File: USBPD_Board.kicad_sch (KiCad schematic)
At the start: 0 parts

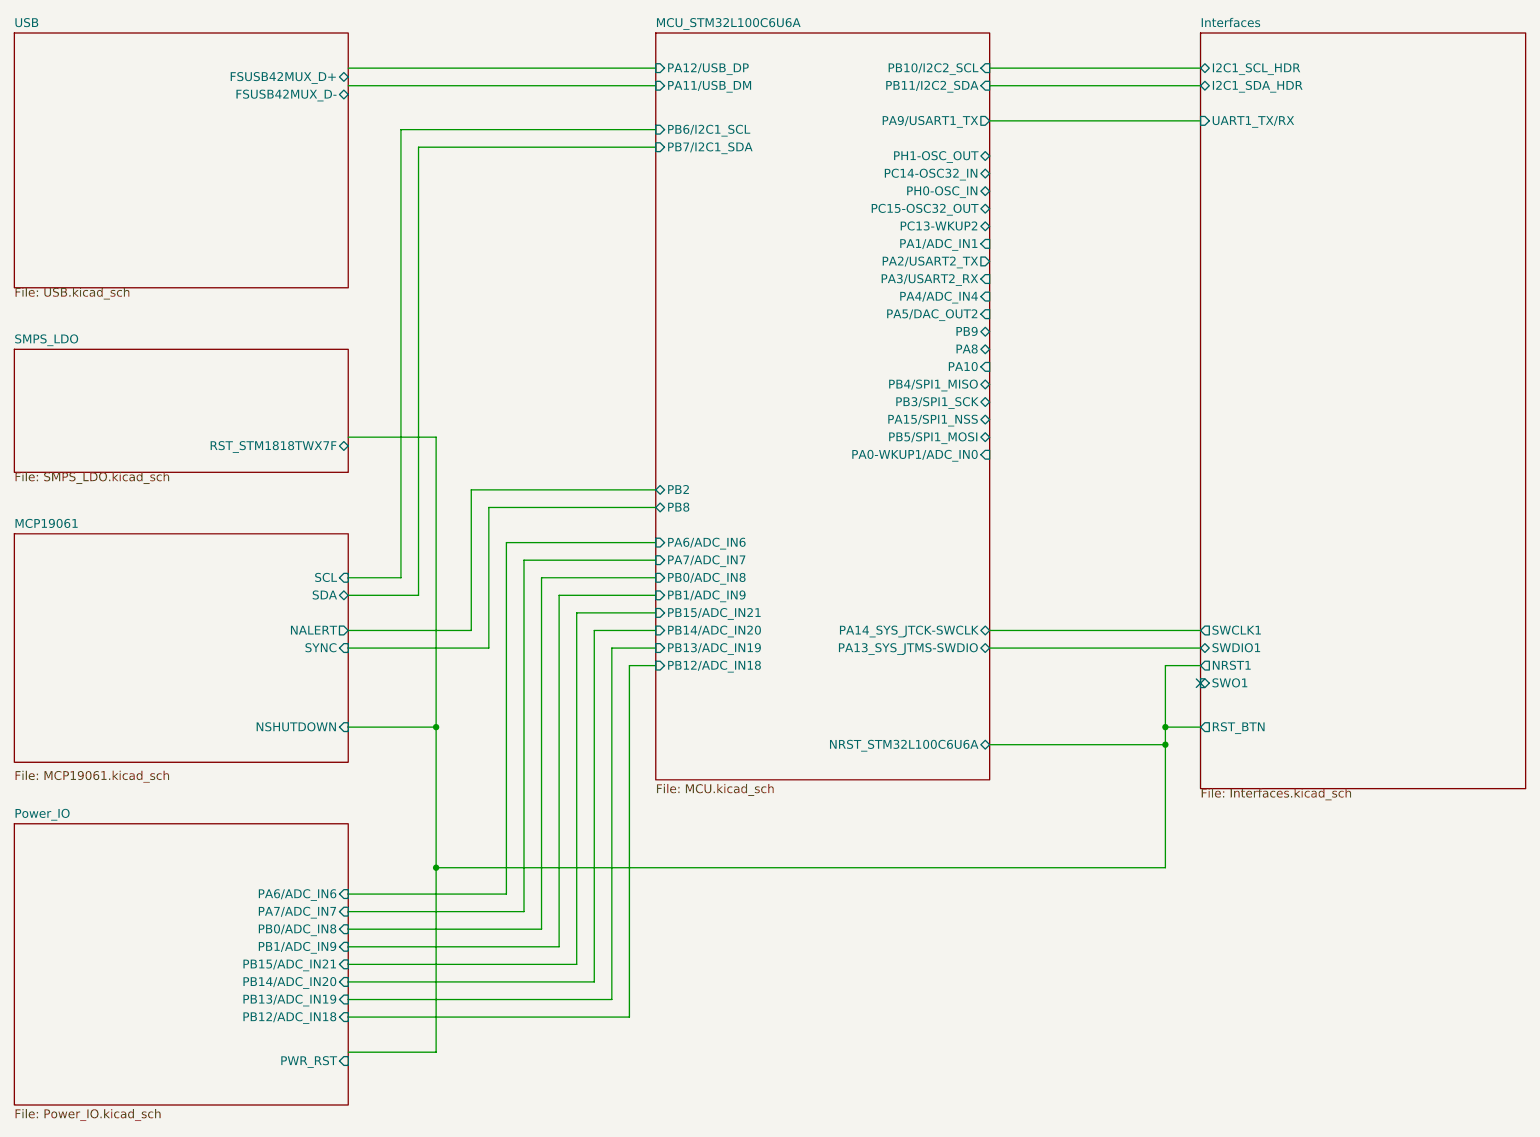
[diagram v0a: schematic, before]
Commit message: Update
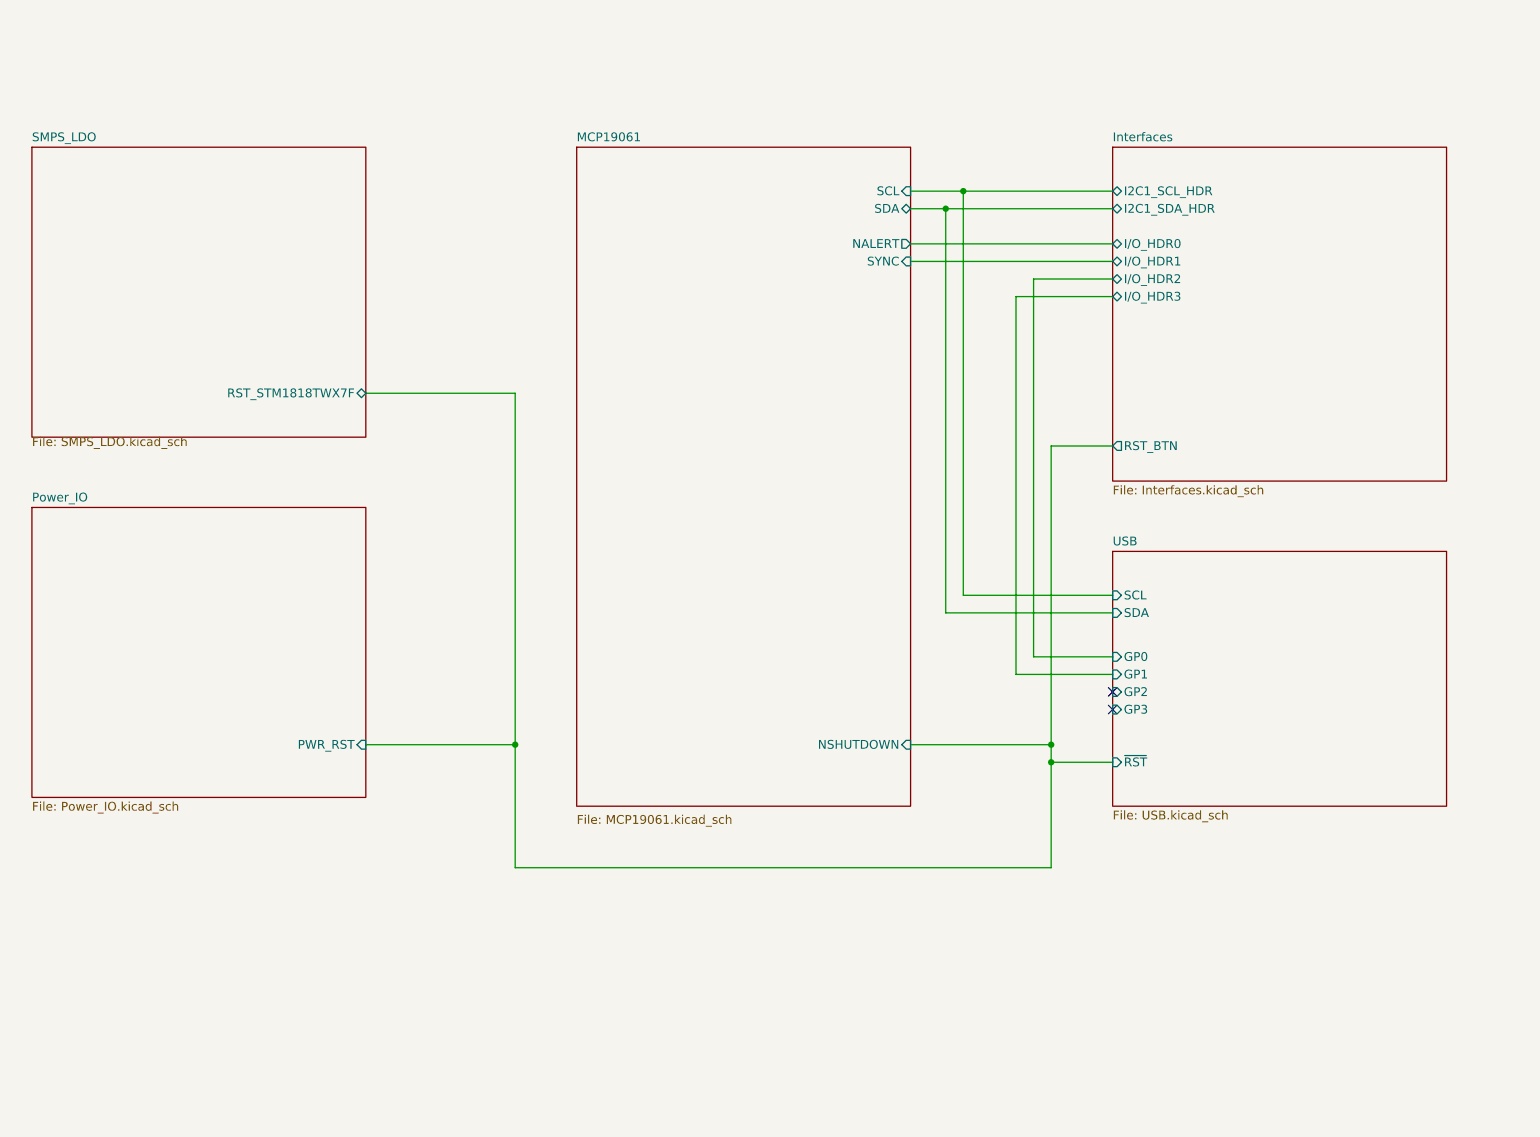
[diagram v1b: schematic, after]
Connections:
- no-connect marks 1 -> 2
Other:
- removed sheet MCU_STM32L100C6U6A
- sheet Interfaces ports: added I/O_HDR0, I/O_HDR1, I/O_HDR2, I/O_HDR3; removed NRST1, SWCLK1, SWDIO1, SWO1, UART1_TX/RX
- sheet Power_IO ports: added none; removed PA6/ADC_IN6, PA7/ADC_IN7, PB0/ADC_IN8, PB12/ADC_IN18, PB13/ADC_IN19, PB14/ADC_IN20, PB15/ADC_IN21, PB1/ADC_IN9
- sheet USB ports: added GP0, GP1, GP2, GP3, SCL, SDA, ~{RST}; removed FSUSB42MUX_D+, FSUSB42MUX_D-

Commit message: Update
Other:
- company: (none) -> Peter Hancak
- title: (none) -> USB-PD Board
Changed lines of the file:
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@@
 	(generator_version "8.0")
 	(paper "USLetter")
+	(title_block
+		(title "USB-PD Board")
+		(date "2025-12-03")
+		(rev "B")
+		(company "Peter Hancak")
+	)
 	(junction
 		(at 184.15 133.35)
